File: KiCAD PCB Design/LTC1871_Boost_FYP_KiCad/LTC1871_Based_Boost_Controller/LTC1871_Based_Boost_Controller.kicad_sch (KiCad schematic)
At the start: 1 part, among them U1 LTC1871EMS-7-PBF

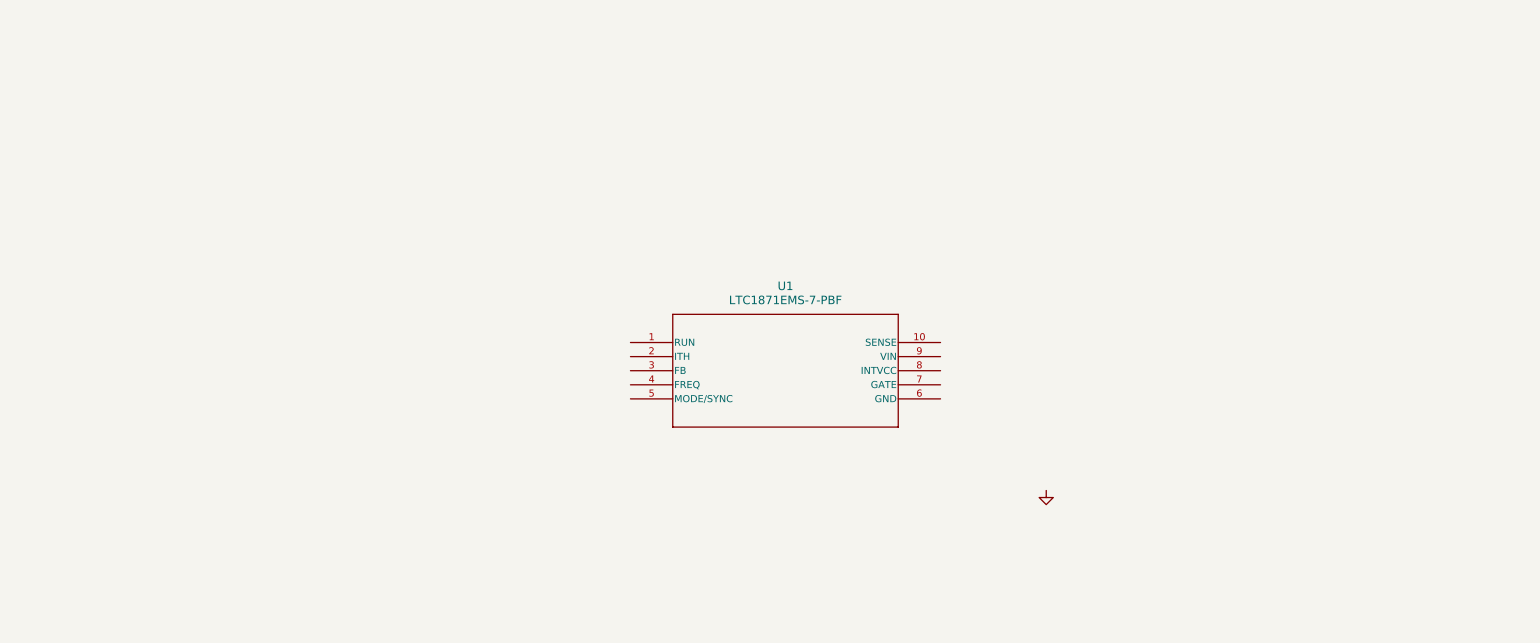
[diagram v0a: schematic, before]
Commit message: Auto-sync from Fortune at 2026-04-08 13:10:18
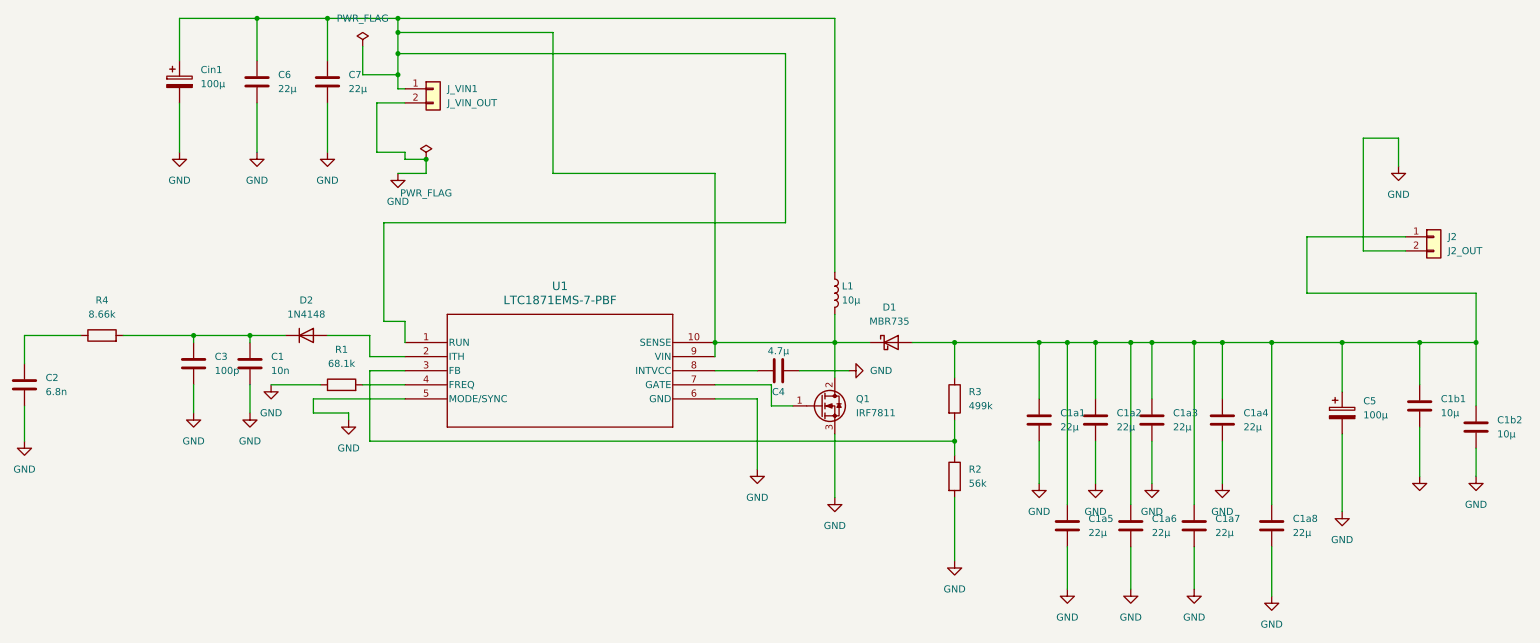
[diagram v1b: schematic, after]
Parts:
- added C1: 10n, Capacitor_SMD:C_0805_2012Metric, symbol Device:C
- added C1a1, C1a2, C1a3, C1a4, C1a5, C1a6, C1a7, C1a8, C6, C7: 22µ, Capacitor_SMD:C_1206_3216Metric, symbol Device:C
- added C1b1, C1b2: 10µ, Capacitor_SMD:C_0805_2012Metric, symbol Device:C
- added C2: 6.8n, Capacitor_SMD:C_0805_2012Metric, symbol Device:C
- added C3: 100p, Capacitor_SMD:C_0805_2012Metric, symbol Device:C
- added C4: 4.7µ, Capacitor_SMD:C_0805_2012Metric, symbol Device:C
- added C5, Cin1: 100µ, Capacitor_THT:CP_Radial_D8.0mm_P3.50mm, symbol Device:C_Polarized
- added D1: MBR735, Diode_THT:D_DO-201AD_P15.24mm_Horizontal, symbol Device:D_Schottky
- added D2: 1N4148, Diode_SMD:D_SOD-323_HandSoldering, symbol Device:D
- added J2: J2_OUT, symbol Connector_Generic:Conn_01x02
- added J_VIN1: J_VIN_OUT, Connector_PinHeader_2.54mm:PinHeader_1x02_P2.54mm_Vertical, symbol Connector_Generic:Conn_01x02
- added L1: 10µ, Inductor_SMD:L_Coilcraft_XAL6060-XXX, symbol Device:L
- added Q1: IRF7811, Package_SO:SOIC-8_3.9x4.9mm_P1.27mm, symbol Transistor_FET:Q_NMOS_GDS
- added R1: 68.1k, Resistor_SMD:R_0805_2012Metric, symbol Device:R
- added R2: 56k, Resistor_SMD:R_0805_2012Metric, symbol Device:R
- added R3: 499k, Resistor_SMD:R_0805_2012Metric, symbol Device:R
- added R4: 8.66k, Resistor_SMD:R_0805_2012Metric, symbol Device:R
- U1: footprint MSOP-10_MS_LIT -> Package_SO:MSOP-10_3x3mm_P0.5mm
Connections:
- net GND: now also U1.5 (MODE/SYNC), U1.6 (GND), C1.2, C1a1.2, C1a2.2, C1a3.2, C1a4.2, C1a5.2, C1a6.2, C1a7.2, C1a8.2, C1b1.2, C1b2.2, C2.2, C3.2, C4.2, C5.2, C6.2, C7.2, Cin1.2, J2.2 (Pin_2), J_VIN1.2 (Pin_2), Q1.3 (S), R1.1, R2.2
- net at U1.1 (RUN): now also U1.10 (SENSE), U1.9 (VIN), C6.1, C7.1, Cin1.1, D1.1 (K), J_VIN1.1 (Pin_1), L1.1, L1.2, Q1.2 (D)
- net at U1.2 (ITH): now also D2.2 (A)
- net at U1.3 (FB): now also R2.1, R3.2
- net at U1.4 (FREQ): now also R1.2
- net at U1.7 (GATE): now also Q1.1 (G)
- net at U1.8 (INTVCC): now also C4.1
- new net: C1a1.1, C1a2.1, C1a3.1, C1a4.1, C1a5.1, C1a6.1, C1a7.1, C1a8.1, C1b1.1, C1b2.1, C5.1, D1.2 (A), J2.1 (Pin_1), R3.1
- new net: C1.1, C3.1, D2.1 (K), R4.2
- new net: C2.1, R4.1
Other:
- moved on the sheet: U1
